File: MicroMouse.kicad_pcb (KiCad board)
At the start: 2 copper layers, 100 x 80 mm, 83 parts, among them CN1 mouseBattery, Q1 IRLML6402, Q2 IRLML6344, U1 STM32F405RGTx, U2 TB6612, U3 CN_MOTOR, U4 CN_MOTOR, U5 3p, U6 ICM-20602, U7 4p

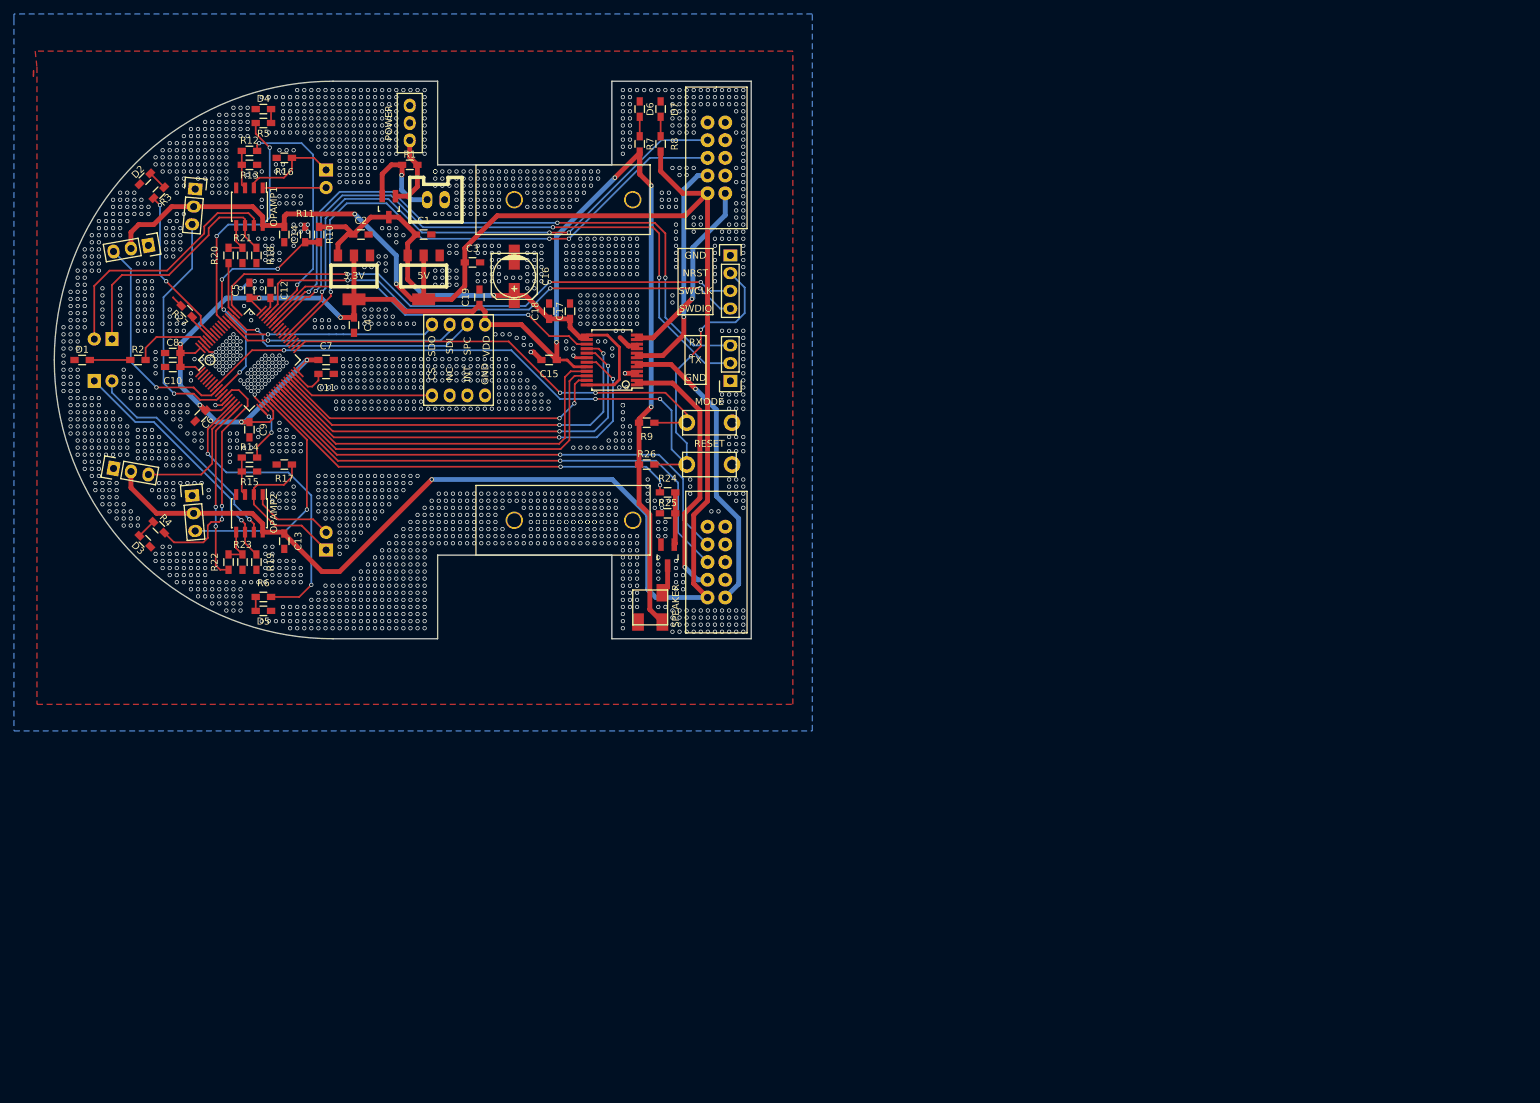
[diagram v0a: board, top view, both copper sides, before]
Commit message: 発注した
何かあったら回路図修正に戻ること
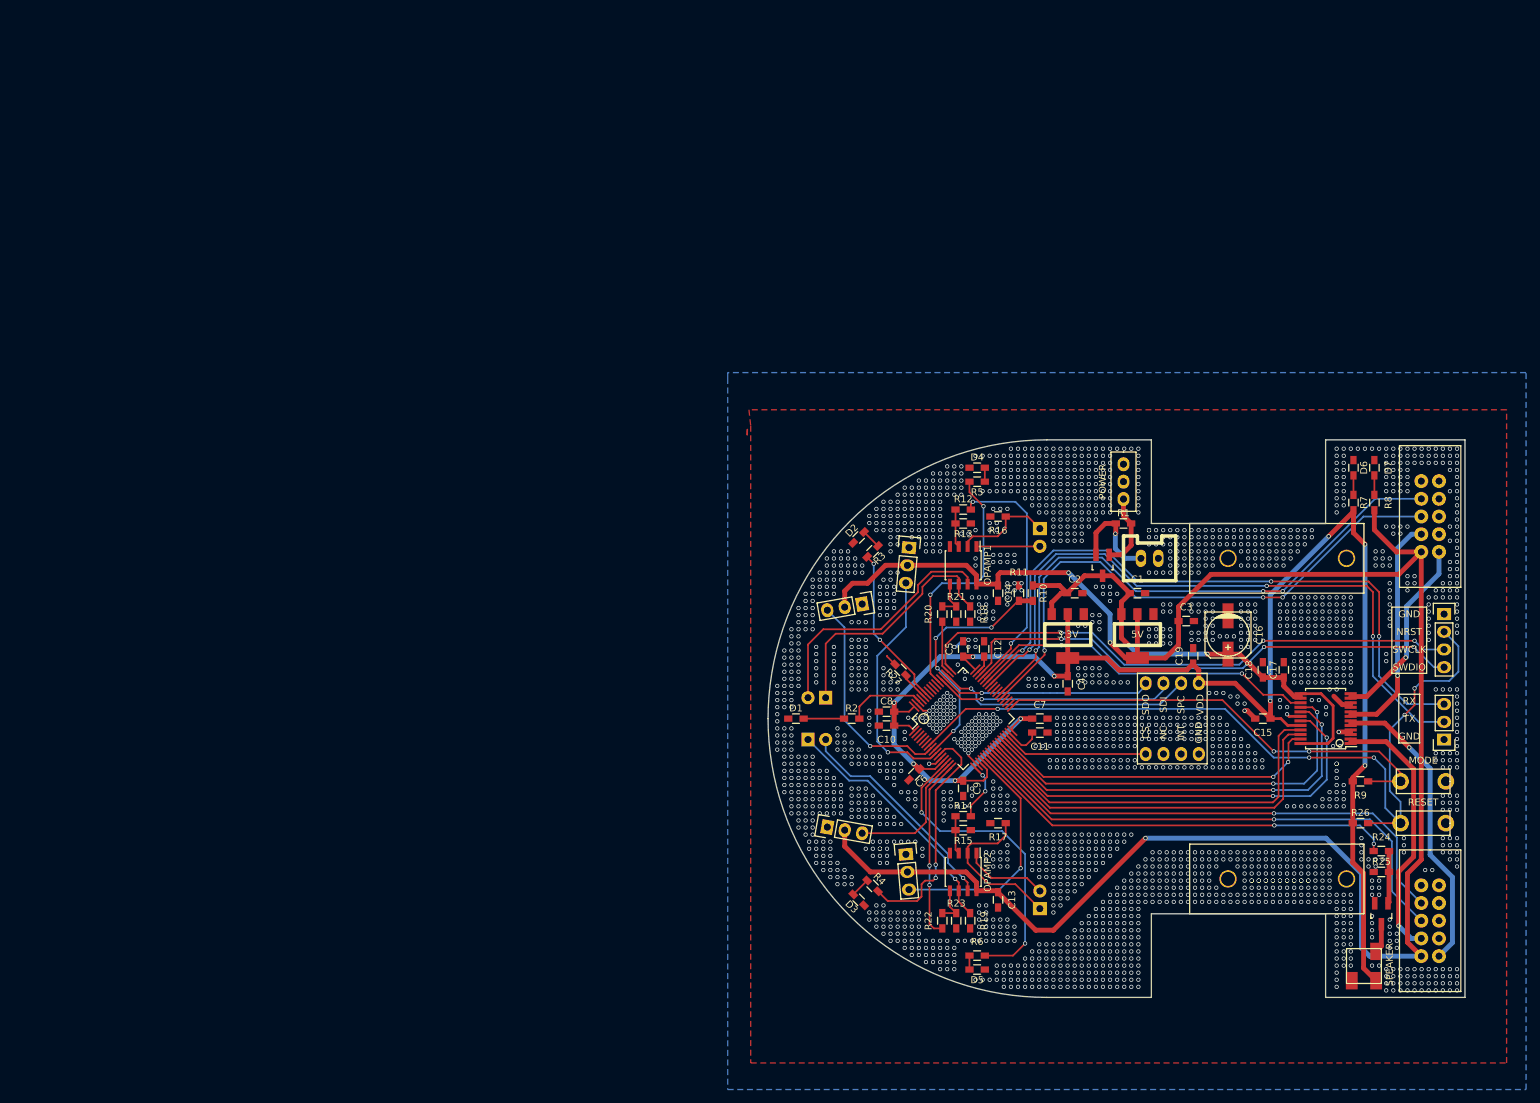
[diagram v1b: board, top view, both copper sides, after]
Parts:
- moved 3.3V 114.6 mm to (145.4, 76.5)
- moved 5V 114.6 mm to (155.4, 76.5)
- moved C1 114.6 mm to (155.4, 73.5)
- moved C10 114.6 mm to (119.4, 92.5)
- moved C11 114.6 mm to (141.4, 93.5)
- moved C12 114.6 mm to (133.4, 81.5)
- moved C13 114.6 mm to (135.4, 117.5)
- moved C14 114.6 mm to (135.4, 73.5)
- moved C15 114.6 mm to (173.4, 91.5)
- moved C16 114.6 mm to (168.4, 79.5)
- moved C17 114.6 mm to (176.4, 84.5)
- moved C18 114.6 mm to (173.4, 84.5)
- moved C19 114.6 mm to (163.4, 82.5)
- moved C2 114.6 mm to (146.4, 73.5)
- moved C3 114.6 mm to (162.4, 77.5)
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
